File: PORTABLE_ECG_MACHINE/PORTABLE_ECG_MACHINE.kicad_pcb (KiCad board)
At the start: 2 copper layers, 75 parts, among them IC1 AD8232ACPZ, J1 UART, J2 Li-Ion 3.7 CONN, J3 USB_B_Micro, Q1 BSS138, Q2 BSS138, SW1 SW_SPDT, U1 SSD1306, U2 CP2102-GM, U3 TC1262-33, U4 TP4056

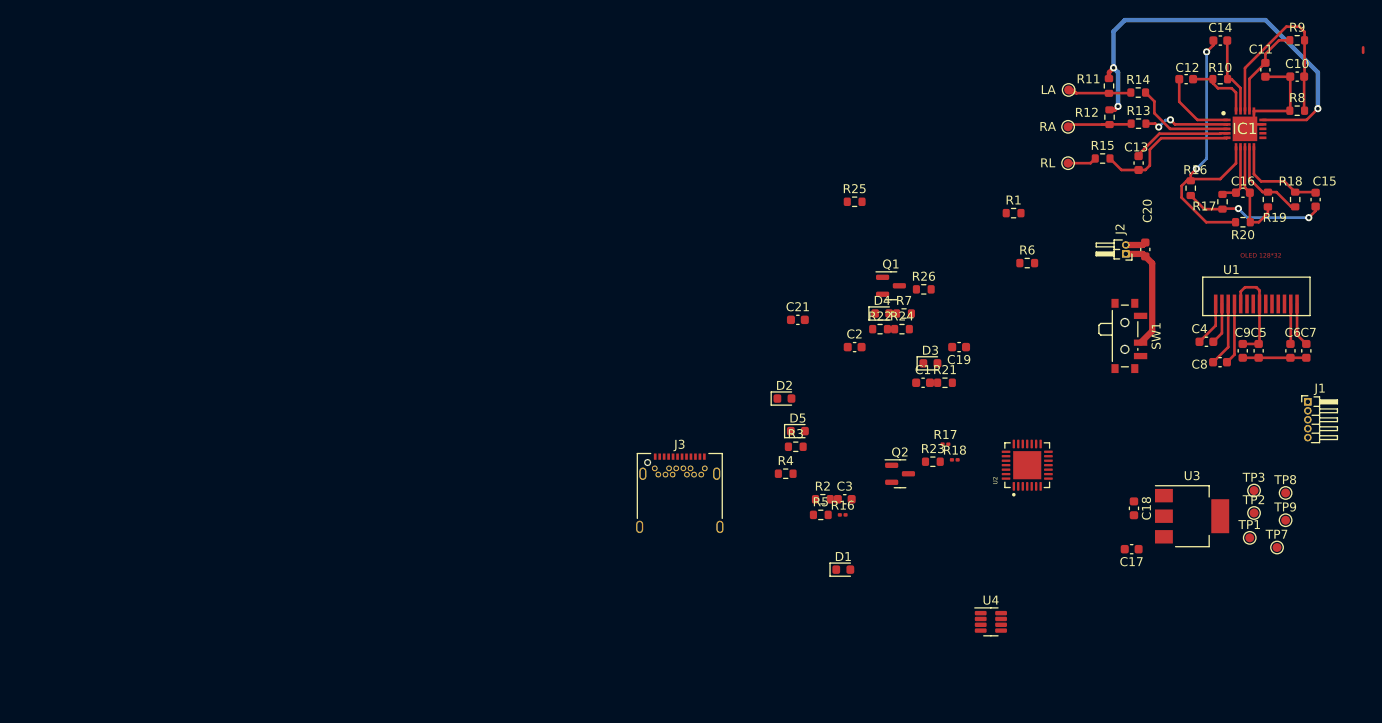
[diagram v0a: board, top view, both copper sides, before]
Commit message: PCBNEW ROUGH STRUCTURE | EDGECUT PR
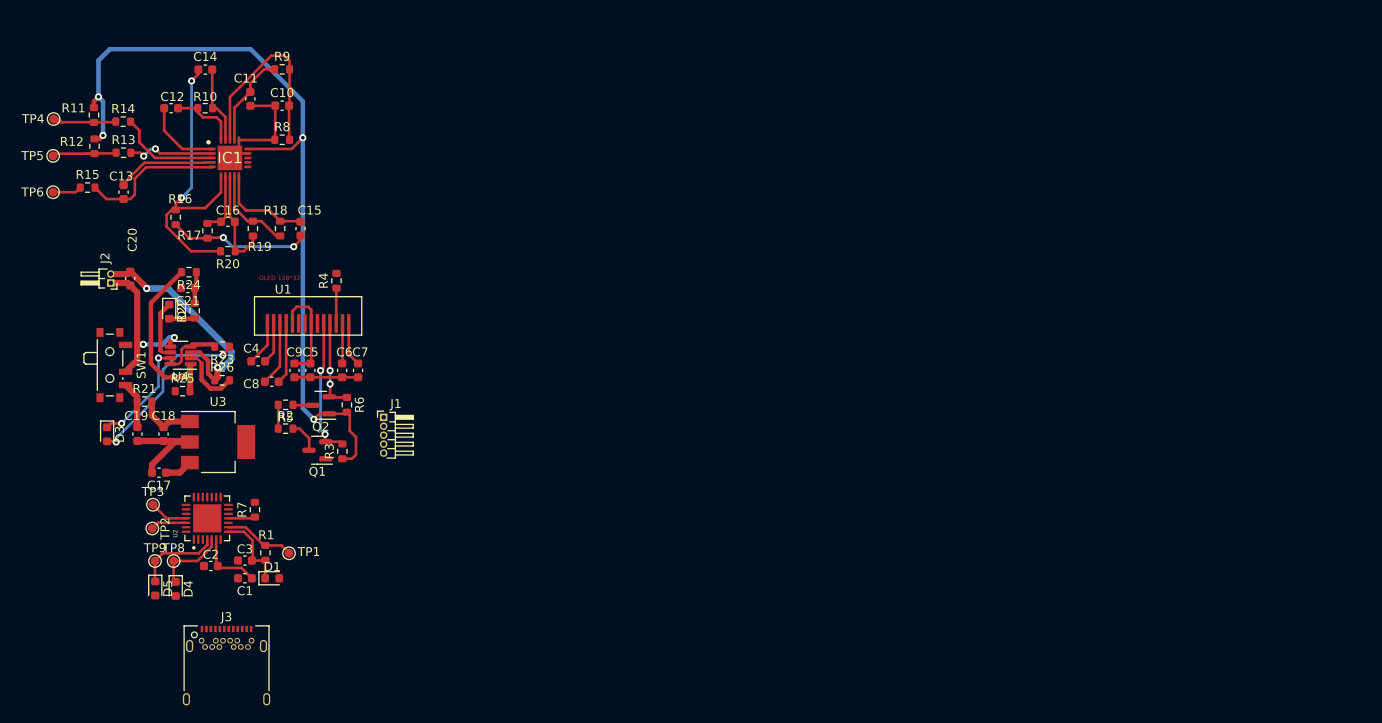
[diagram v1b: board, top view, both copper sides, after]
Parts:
- removed the R16 at (165.5, 73.1)
- removed the R17 at (177.0, 65.2)
- removed the R18 at (178.1, 67.0)
- removed TP7: B-TEMP, TestPoint:TestPoint_Pad_D1.0mm
- moved TP9 126.5 mm to (88.6, 78.3)
- moved TP8 124.6 mm to (90.7, 78.3)
- moved TP2 123.3 mm to (88.3, 74.7), turned to -90 degrees
- moved TP3 123.2 mm to (88.4, 72.0)
- moved C11 113.6 mm to (99.3, 26.6)
- moved C16 113.6 mm to (96.8, 40.3)
- moved IC1 113.6 mm to (97.0, 33.2)
- moved R12 113.6 mm to (81.9, 31.9)
- moved R17 113.6 mm to (94.5, 41.4)
- moved R20 113.6 mm to (96.8, 43.6)
- moved TP4 113.6 mm to (77.3, 28.8)
- moved C10 113.6 mm to (102.8, 27.4)
- moved C13 113.6 mm to (85.1, 37.0)
- moved C14 113.6 mm to (94.2, 23.3)
- moved C15 113.6 mm to (104.9, 41.1)
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- renumbered LA to TP4, RA to TP5, RL to TP6
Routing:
- net 3.3V: track 47.7 -> 90.6 mm, vias 3 -> 4
- net GND: track 25.3 -> 61.1 mm, vias 0 -> 2
- net Net-(D3-Pad2): track 0.00 -> 19.9 mm, vias 0 -> 2
- net Net-(R24-Pad2): track 0.00 -> 19.6 mm
- net SCL_3.3: track 0.00 -> 15.7 mm, vias 0 -> 2
- net Net-(D3-Pad1): track 0.00 -> 12.2 mm, vias 0 -> 2
- net SDA_3.3: track 0.00 -> 10.3 mm, vias 0 -> 2
- net Net-(C21-Pad1): track 0.00 -> 10.0 mm
- net USB_D-: track 0.00 -> 9.49 mm
- net VIN: track 0.00 -> 8.95 mm
- net USB_D+: track 0.00 -> 8.16 mm
- net Net-(R1-Pad2): track 0.00 -> 7.74 mm
- net Net-(C1-Pad1): track 0.00 -> 7.42 mm
- net Net-(R26-Pad2): track 0.00 -> 7.21 mm
- net Net-(D2-Pad1): track 0.00 -> 6.74 mm
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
